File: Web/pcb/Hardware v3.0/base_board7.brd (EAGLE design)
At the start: 80.3 x 80.3 mm, 145 parts, among them IC1 LM2596S, IC2A TDA2822D, IC2B LM386M-1, IC3 TJA1040T, IC4 STM32F103RBT6, IC5 MIC2288BML, IC6 ULN2003AD, IC7 LM2901M, IC8 REG1117, IC9A SN74LVC1G10DCKR, IC9B SN74HC10D, Q1 CSM-7X-DU

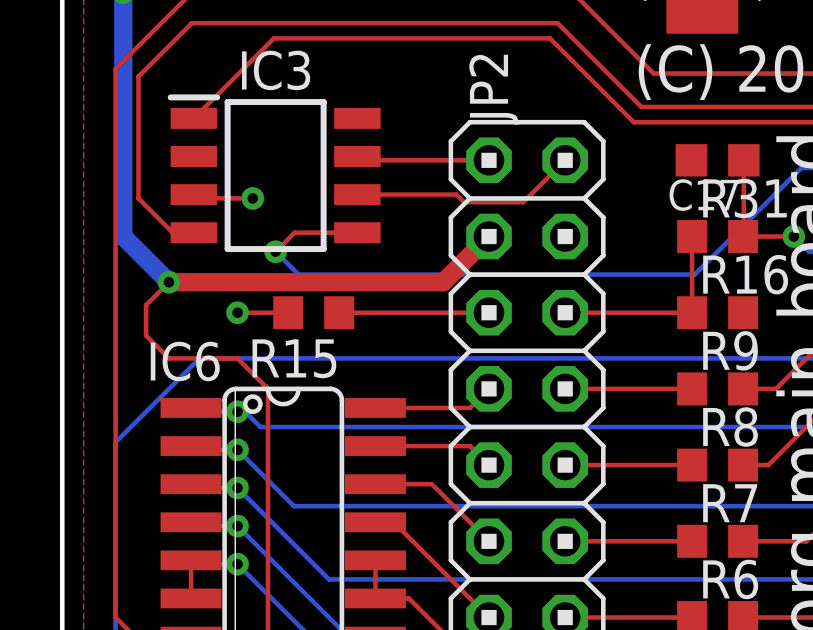
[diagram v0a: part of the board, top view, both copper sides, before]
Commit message: ui updates
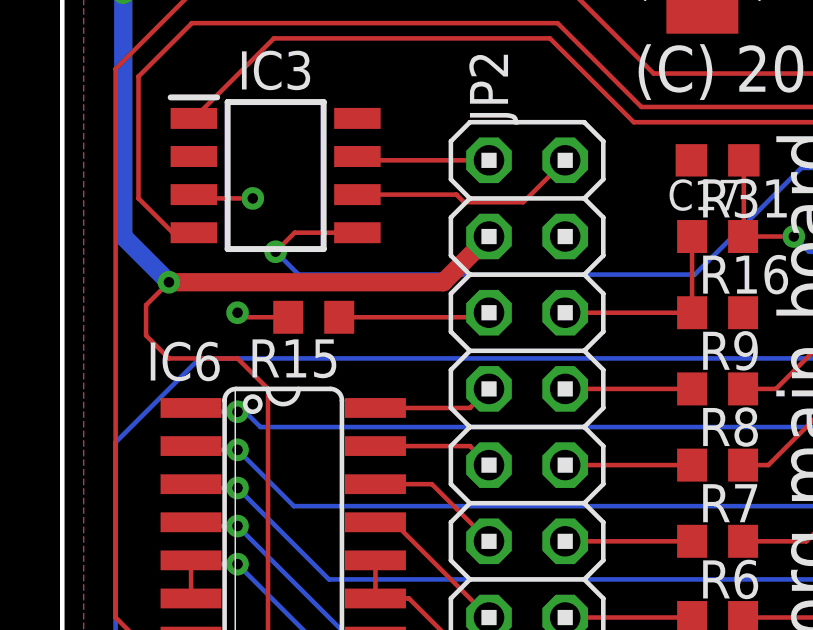
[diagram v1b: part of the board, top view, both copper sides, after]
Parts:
- moved R15 0.15 mm to (-36.3, 12.5)
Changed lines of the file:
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@@
 <attribute name="VALUE" x="-7.15" y="12.32" size="1.016" layer="27"/>
 </element>
-<element name="R15" library="rcl" library_urn="urn:adsk.eagle:library:334" package="R0603" package3d_urn="urn:adsk.eagle:package:23555/2" value="510" x="-36.322" y="12.7" smashed="yes" rot="R180">
+<element name="R15" library="rcl" library_urn="urn:adsk.eagle:library:334" package="R0603" package3d_urn="urn:adsk.eagle:package:23555/2" value="510" x="-36.322" y="12.5476" smashed="yes" rot="R180">
 <attribute name="NAME" x="-35.433" y="11.811" size="1.27" layer="25" rot="R180"/>
-<attribute name="SPICEPREFIX" value="R" x="-36.322" y="12.7" size="1.778" layer="27" rot="R180" display="off"/>
-<attribute name="VALUE" x="-35.687" y="14.605" size="1.27" layer="27" rot="R180"/>
+<attribute name="SPICEPREFIX" value="R" x="-36.322" y="12.5476" size="1.778" layer="27" rot="R180" display="off"/>
+<attribute name="VALUE" x="-35.687" y="14.4526" size="1.27" layer="27" rot="R180"/>
 </element>
 <element name="R31" library="rcl" library_urn="urn:adsk.eagle:library:334" package="R0603" package3d_urn="urn:adsk.eagle:package:23555/2" value="10k" x="-22.86" y="15.24" smashed="yes">
@@
 <wire x1="-20.32" y1="-15.24" x2="-22.01" y2="-15.24" width="0.1524" layer="1"/>
 <via x="-38.862" y="12.7" extent="1-16" drill="0.35"/>
-<wire x1="-37.172" y1="12.7" x2="-38.862" y2="12.7" width="0.1524" layer="1"/>
+<wire x1="-37.172" y1="12.5476" x2="-38.7096" y2="12.5476" width="0.1524" layer="1"/>
+<wire x1="-38.7096" y1="12.5476" x2="-38.862" y2="12.7" width="0.1524" layer="1"/>
 <via x="-38.354" y="16.51" extent="1-16" drill="0.35"/>
 <wire x1="-38.354" y1="16.51" x2="-40.19" y2="16.51" width="0.1524" layer="1"/>
@@
 <contactref element="JP2" pad="22"/>
 <contactref element="R15" pad="1"/>
-<wire x1="-35.472" y1="12.7" x2="-30.48" y2="12.7" width="0.1524" layer="1"/>
+<wire x1="-30.6324" y1="12.5476" x2="-30.48" y2="12.7" width="0.1524" layer="1"/>
+<wire x1="-30.6324" y1="12.5476" x2="-35.472" y2="12.5476" width="0.1524" layer="1"/>
 </signal>
 <signal name="CANH">
